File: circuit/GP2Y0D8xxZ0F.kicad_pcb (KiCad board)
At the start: 2 copper layers, 26.8 x 24.9 mm, 13 parts, among them P1 CONN_01X04, U1 GP2Y0D81xZ0F

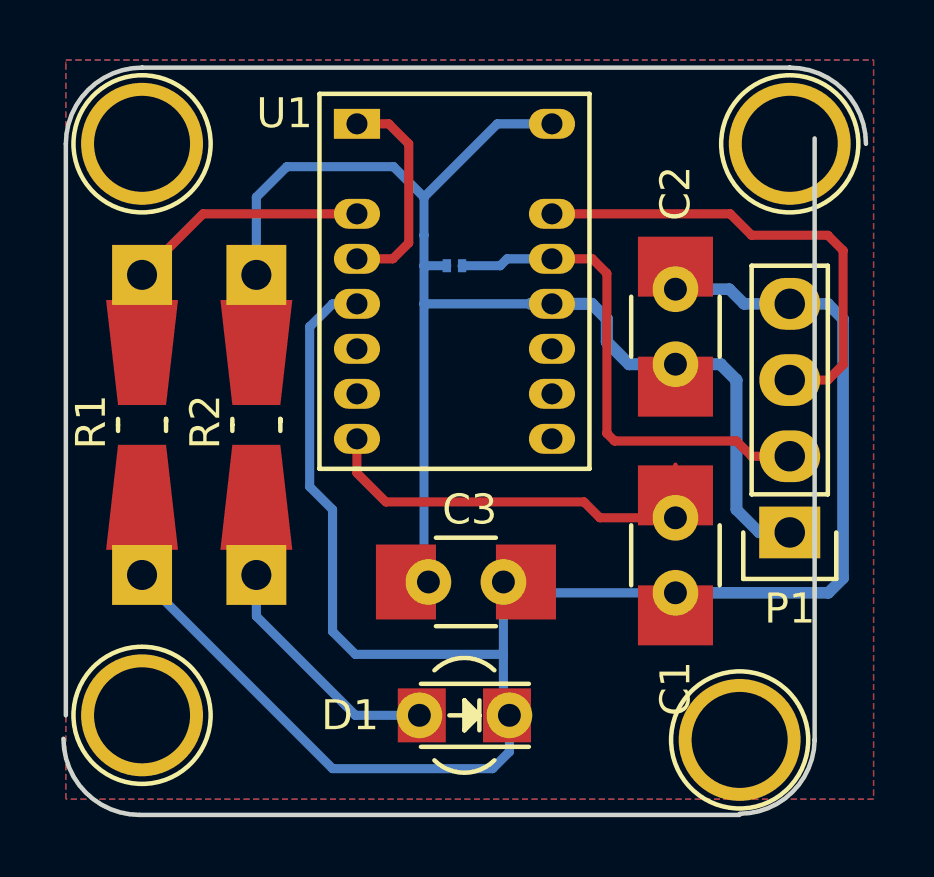
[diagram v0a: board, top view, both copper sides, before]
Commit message: changes in progress, open project with version 5 of kicad and the resizing started
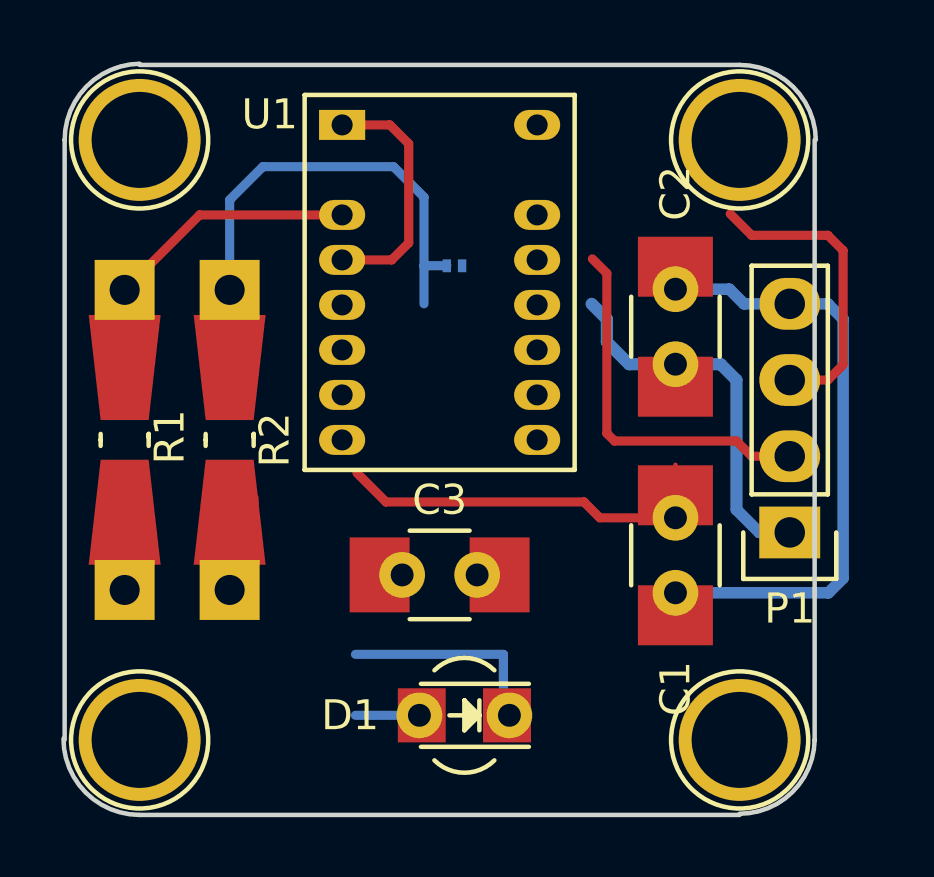
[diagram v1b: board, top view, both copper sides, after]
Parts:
- moved REF** 1.68 mm to (91.0, 78.5)
- moved R2 1.02 mm to (74.0, 88.5)
- moved C3 0.91 mm to (81.0, 93.0)
- moved REF** 0.82 mm to (71.0, 98.5)
- moved R1 0.77 mm to (70.5, 88.5)
- moved U1 0.50 mm to (81.0, 84.0)
- moved REF** 0.15 mm to (71.0, 78.5)
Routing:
- net GND: track 70.0 -> 31.1 mm
- net VCC: track 50.8 -> 30.5 mm
- net Net-(D1-Pad2): track 10.8 -> 4.72 mm
- net /Output: track 16.0 -> 10.1 mm
- net /Enable: track 17.6 -> 13.2 mm
- net Net-(C1-Pad1): track 15.0 -> 13.9 mm
- removed copper zone on B.Cu, net GND
- removed copper zone on F.Cu, net GND
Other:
- board size 26.8 x 24.9 mm -> 25.1 x 25 mm
